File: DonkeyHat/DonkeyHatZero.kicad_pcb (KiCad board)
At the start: 2 copper layers, 66.2 x 29.2 mm, 12 parts, among them J1 GPIO, J2 Conn_01x02_Pin, J3 Conn_01x02_Pin, J5 Battery +, J6 Battery -, J7 +5v, J8 GND, U2 rp2040-zero

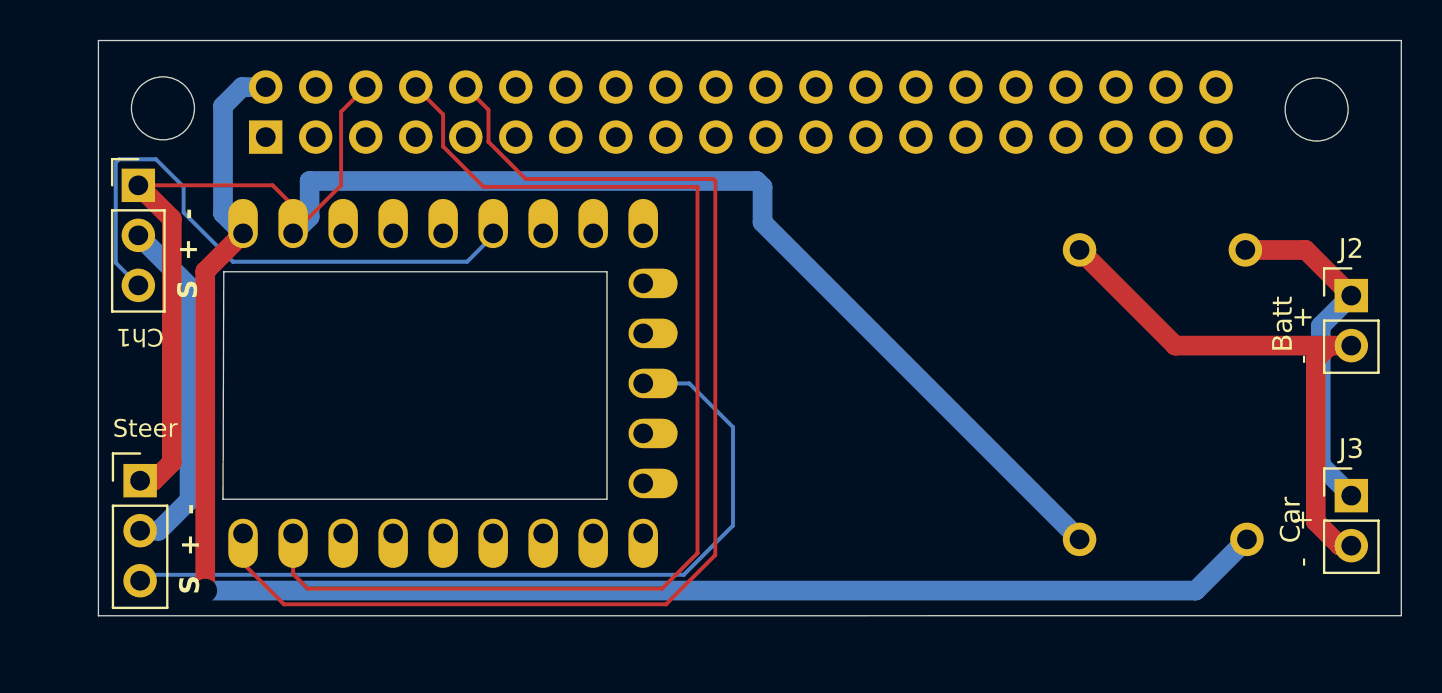
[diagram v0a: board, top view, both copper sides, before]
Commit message: Updated zero
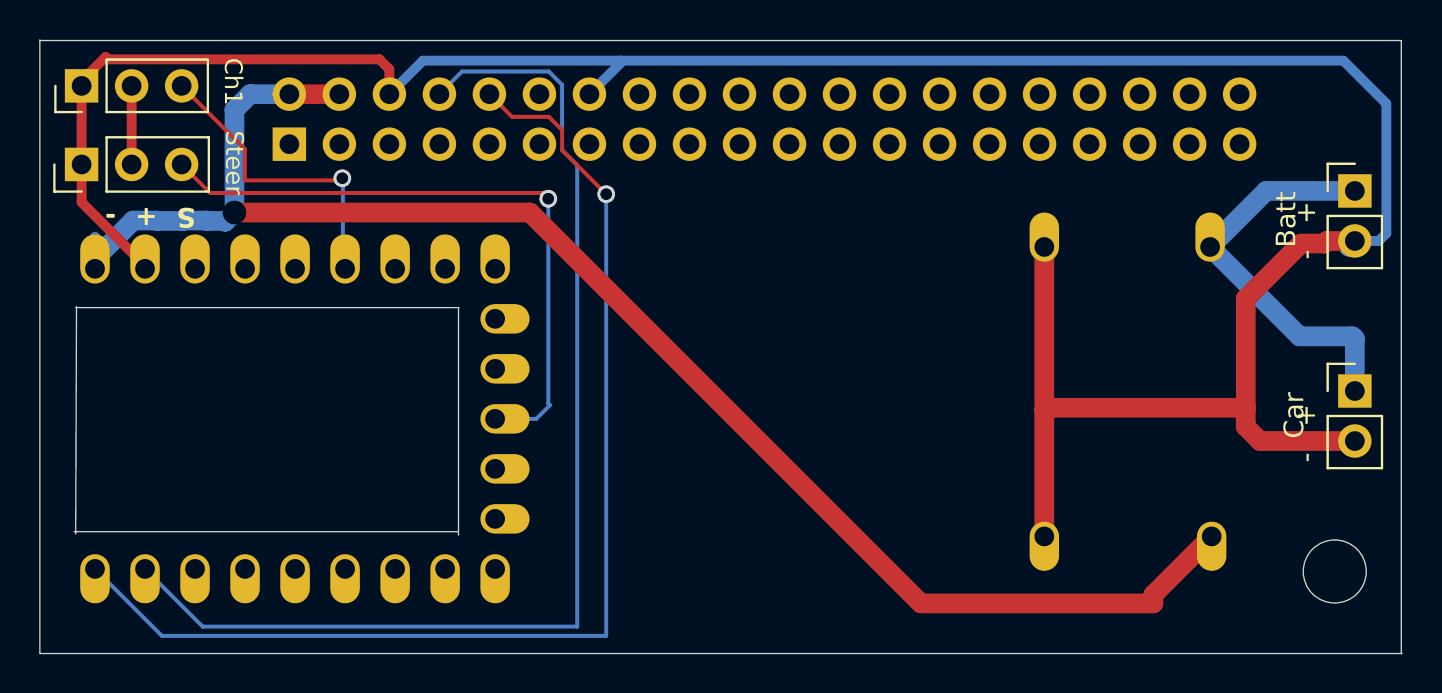
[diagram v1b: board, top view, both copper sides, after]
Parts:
- removed J5: Battery +, Connector_PinHeader_2.54mm:PinHeader_1x01_P2.54mm_Vertical
- removed J6: Battery -, Connector_PinHeader_2.54mm:PinHeader_1x01_P2.54mm_Vertical
- removed J7: +5v, Connector_PinHeader_2.54mm:PinHeader_1x01_P2.54mm_Vertical
- removed J8: GND, Connector_PinHeader_2.54mm:PinHeader_1x01_P2.54mm_Vertical
- removed the REF** at (103.2, 47.3)
- added ?: , , F.Cu at (147.9, 69.0)
- added ?: , , F.Cu at (156.3, 54.4)
- added ?: , , F.Cu at (147.9, 54.4)
- added ?: , , F.Cu at (156.4, 69.0)
- moved REF** 23.5 mm to (162.7, 70.8)
- moved Steer1 16.3 mm to (99.0, 50.2), turned to 90 degrees
- moved U2 7.73 mm to (109.9, 63.1)
- moved RCin1 5.81 mm to (99.0, 46.2), turned to 90 degrees
- moved J3 5.32 mm to (163.7, 61.7)
- moved J2 5.32 mm to (163.7, 51.5)
- moved J1 1.25 mm to (109.6, 49.1)
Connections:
- J2 pad 1: Net-(J2-Pin_1) -> Batt
- J2 pad 2: Net-(J2-Pin_2) -> GND
- J3 pad 1: Net-(J2-Pin_1) -> Batt
- J3 pad 2: Net-(J2-Pin_2) -> GND
- RCin1 pad 2: Batt -> Net-(RCin1-Pin_2)
- Steer1 pad 2: Batt -> Net-(RCin1-Pin_2)
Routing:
- net GND: track 86.1 -> 136.0 mm
- net Net-(J2-Pin_2): track 27.3 -> 0.00 mm
- net Net-(J2-Pin_1): track 17.8 -> 0.00 mm
- net RCin1: track 29.5 -> 15.4 mm, vias 0 -> 1
- net Steer: track 41.7 -> 33.1 mm, vias 0 -> 1
- net Net-(RCin1-Pin_2): track 0.00 -> 3.99 mm
- net Rpi Rx: track 62.0 -> 58.4 mm, vias 0 -> 1
- net Batt: track 17.7 -> 20.5 mm
- net +5V: track 82.4 -> 80.7 mm
- net Rpi Tx: track 59.6 -> 58.0 mm
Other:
- board size 66.2 x 29.2 mm -> 69.2 x 31.2 mm
